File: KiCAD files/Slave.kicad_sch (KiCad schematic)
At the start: 11 parts, among them U5 NUCLEO64-F446RE

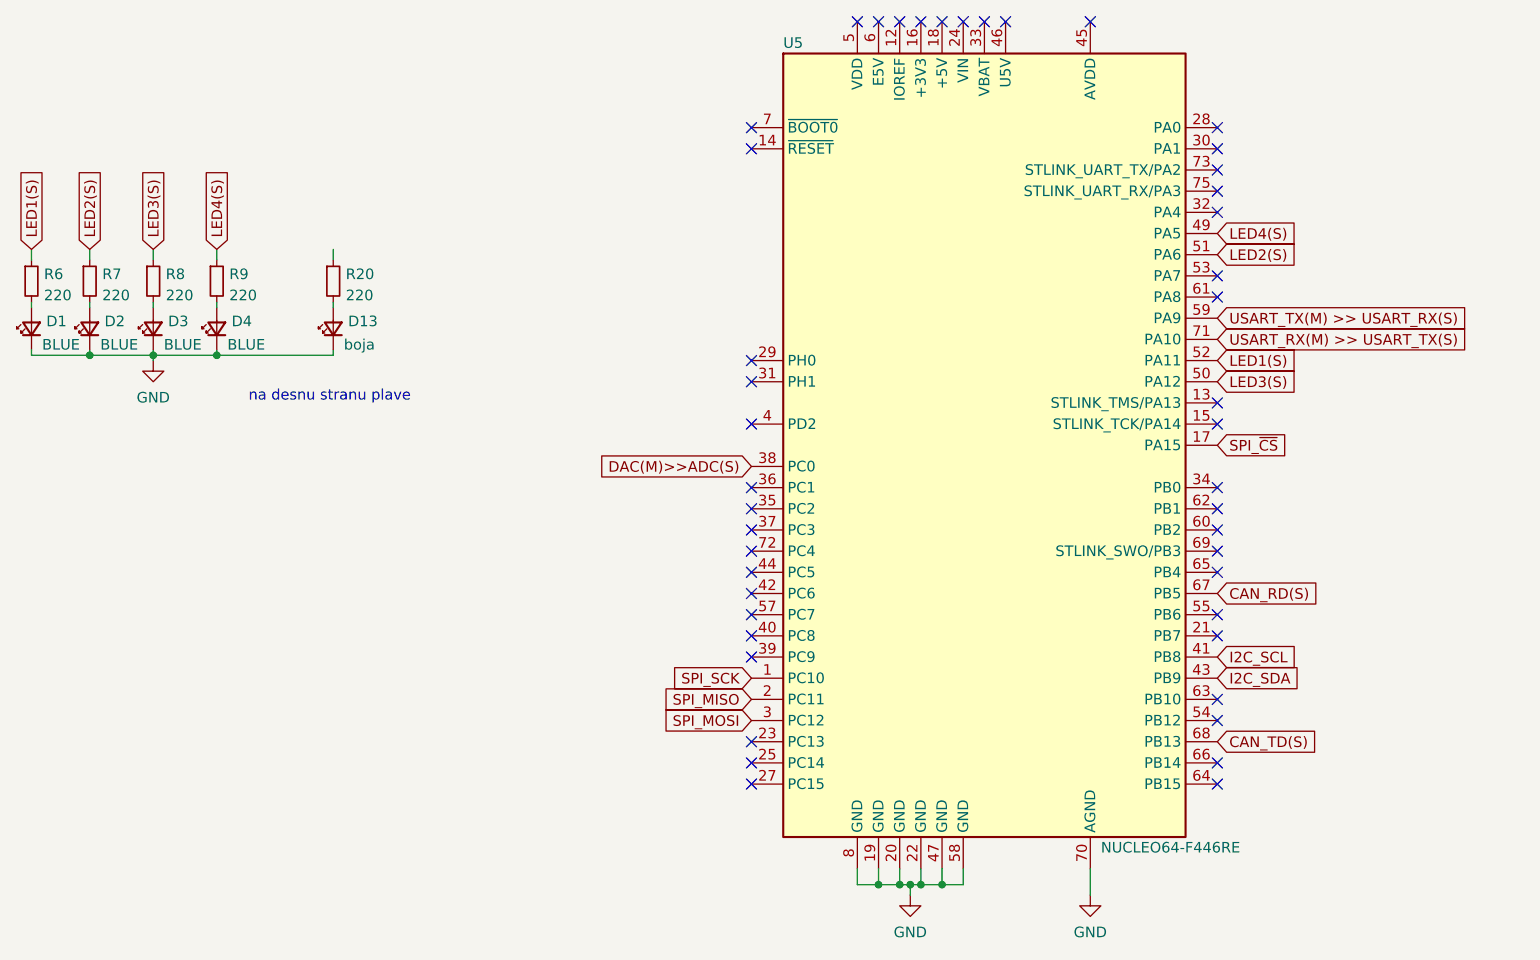
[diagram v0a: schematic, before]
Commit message: update
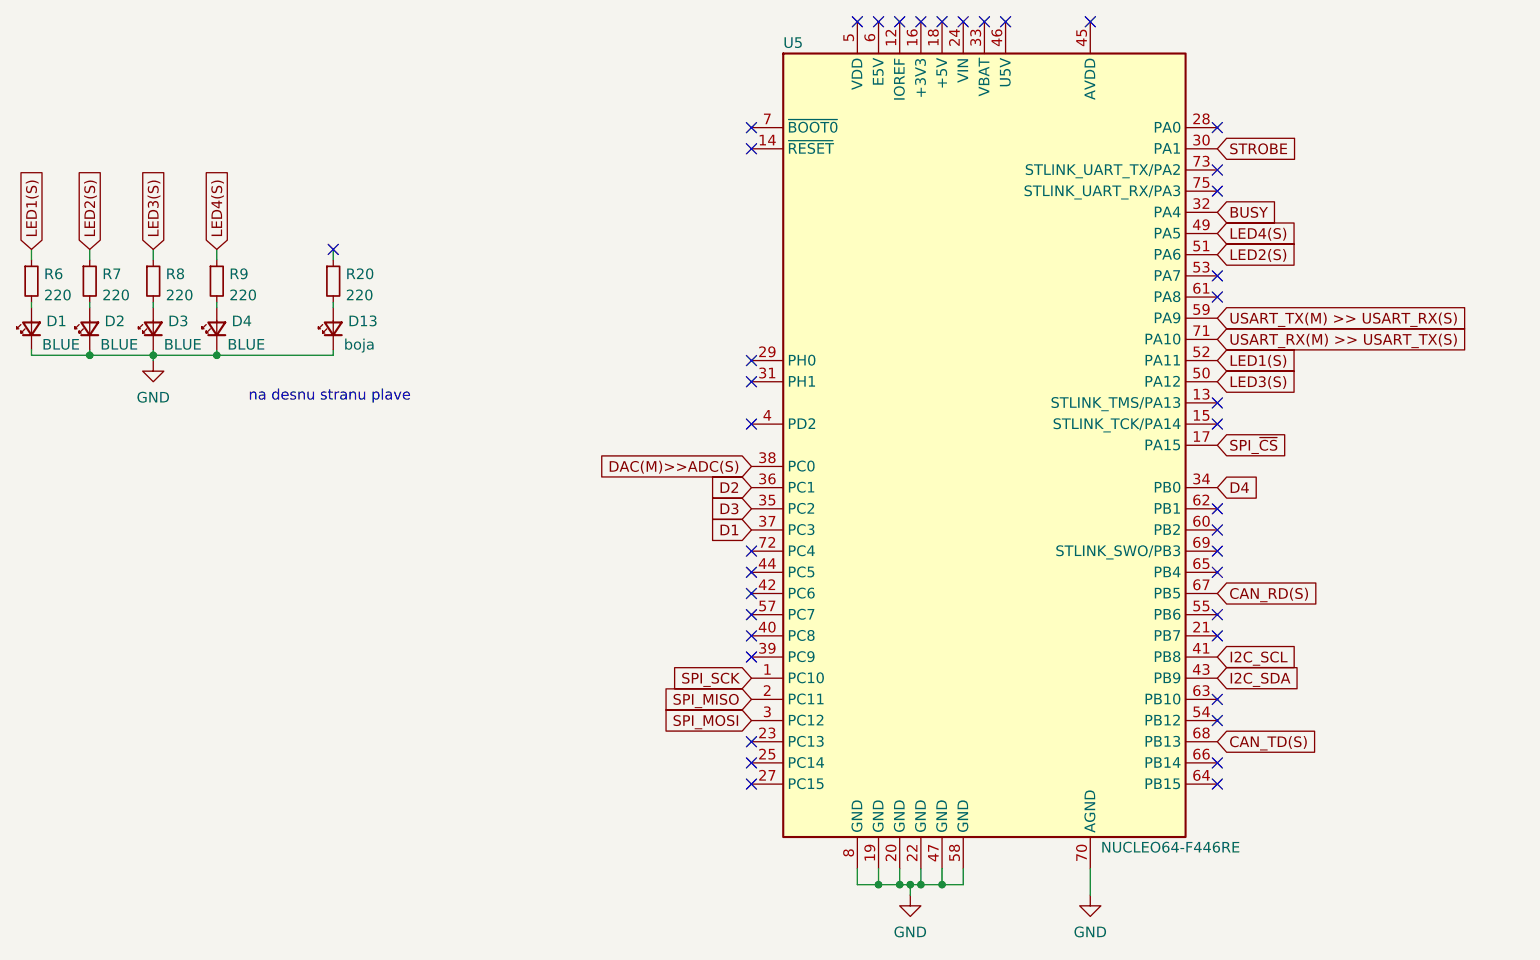
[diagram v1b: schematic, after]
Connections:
- net STROBE: now reaches U5.30 (PA1)
- net BUSY: now reaches U5.32 (PA4)
- net D4: now reaches U5.34 (PB0)
- net D3: now reaches U5.35 (PC2)
- net D2: now reaches U5.36 (PC1)
- net D1: now reaches U5.37 (PC3)
- no-connect marks 46 -> 41
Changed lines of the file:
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@@
   (no_connect (at 142.24 43.18))
   (no_connect (at 157.48 43.18))
-  (no_connect (at 172.72 58.42))
   (no_connect (at 172.72 73.66))
   (no_connect (at 172.72 55.88))
@@
   (no_connect (at 172.72 114.3))
   (no_connect (at 172.72 116.84))
-  (no_connect (at 116.84 104.14))
   (no_connect (at 116.84 116.84))
   (no_connect (at 116.84 55.88))
   (no_connect (at 116.84 119.38))
   (no_connect (at 116.84 129.54))
-  (no_connect (at 172.72 66.04))
+  (no_connect (at 66.675 70.485))
   (no_connect (at 172.72 101.6))
   (no_connect (at 116.84 91.44))
@@
   (no_connect (at 172.72 91.44))
   (no_connect (at 172.72 124.46))
-  (no_connect (at 116.84 99.06))
   (no_connect (at 172.72 60.96))
   (no_connect (at 116.84 114.3))
-  (no_connect (at 172.72 99.06))
-  (no_connect (at 116.84 101.6))
   (no_connect (at 139.7 43.18))
   (no_connect (at 172.72 109.22))
@@
     )
   )
+  (global_label "D2" (shape input) (at 116.84 99.06 180) (fields_autoplaced)
+    (effects (font (size 1.27 1.27)) (justify right))
+    (property "Intersheetrefs" "${INTERSHEET_REFS}" (at 111.3753 99.06 0)
+      (effects (font (size 1.27 1.27)) (justify right) hide)
+    )
+  )
   (global_label "USART_TX(M) >> USART_RX(S)" (shape input) (at 172.72 78.74 0) (fields_autoplaced)
     (effects (font (size 1.27 1.27)) (justify left))
@@
     )
   )
+  (global_label "D1" (shape input) (at 116.84 104.14 180) (fields_autoplaced)
+    (effects (font (size 1.27 1.27)) (justify right))
+    (property "Intersheetrefs" "${INTERSHEET_REFS}" (at 111.3753 104.14 0)
+      (effects (font (size 1.27 1.27)) (justify right) hide)
+    )
+  )
   (global_label "DAC(M)>>ADC(S)" (shape input) (at 116.84 96.52 180) (fields_autoplaced)
     (effects (font (size 1.27 1.27)) (justify right))
@@
     )
   )
+  (global_label "BUSY" (shape input) (at 172.72 66.04 0) (fields_autoplaced)
+    (effects (font (size 1.27 1.27)) (justify left))
+    (property "Intersheetrefs" "${INTERSHEET_REFS}" (at 180.6038 66.04 0)
+      (effects (font (size 1.27 1.27)) (justify left) hide)
+    )
+  )
+  (global_label "STROBE" (shape input) (at 172.72 58.42 0) (fields_autoplaced)
+    (effects (font (size 1.27 1.27)) (justify left))
+    (property "Intersheetrefs" "${INTERSHEET_REFS}" (at 182.9018 58.42 0)
+      (effects (font (size 1.27 1.27)) (justify left) hide)
+    )
+  )
   (global_label "LED2(S)" (shape input) (at 172.72 71.12 0) (fields_autoplaced)
     (effects (font (size 1.27 1.27)) (justify left))
@@
     )
   )
+  (global_label "D4" (shape input) (at 172.72 99.06 0) (fields_autoplaced)
+    (effects (font (size 1.27 1.27)) (justify left))
+    (property "Intersheetrefs" "${INTERSHEET_REFS}" (at 178.1847 99.06 0)
+      (effects (font (size 1.27 1.27)) (justify left) hide)
+    )
+  )
+  (global_label "D3" (shape input) (at 116.84 101.6 180) (fields_autoplaced)
+    (effects (font (size 1.27 1.27)) (justify right))
+    (property "Intersheetrefs" "${INTERSHEET_REFS}" (at 111.3753 101.6 0)
+      (effects (font (size 1.27 1.27)) (justify right) hide)
+    )
+  )
